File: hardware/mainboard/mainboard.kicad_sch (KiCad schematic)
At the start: 124 parts, among them J1 USB 2.0, J10 EXP1, J11 EXP2, J23 JST XH, J24 JST XH, J25 JST XH, J26 JST XH, J27 JST XH, J3 JST XH, J4 JST XH, J5 JST XH, J6 JST XH, J9 Power In, Q1 AGM308MBP, SW13 SW_SPDT, SW14 SW_SPDT, SW2 Reset, SW9 SW_SPDT, U1 STM32F407VGTx, U11 LM5160A, U12 CD40109B, U13 CD40109B, U14 LTV-357T, U15 AMS1117-3.3, U8 LM5160A, U9 CD40109B, Y1 12 MHz

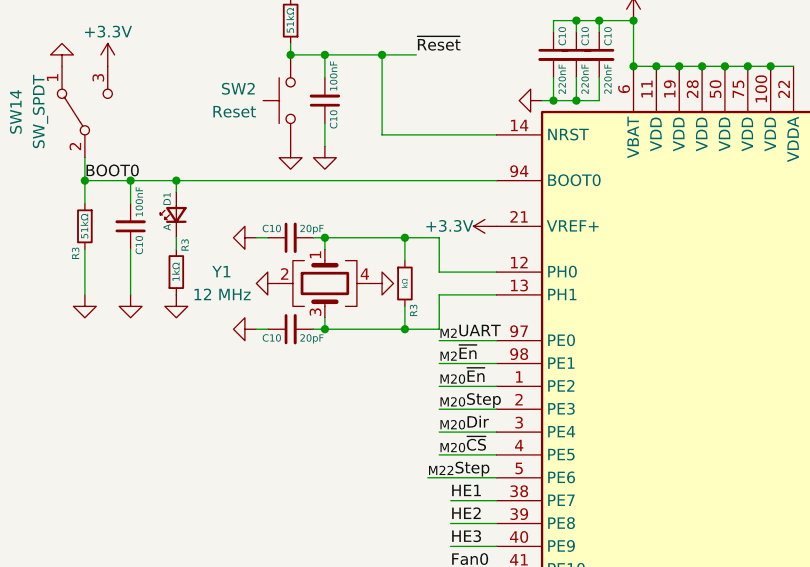
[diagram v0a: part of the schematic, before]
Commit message: test new gitignore with completed mainboard
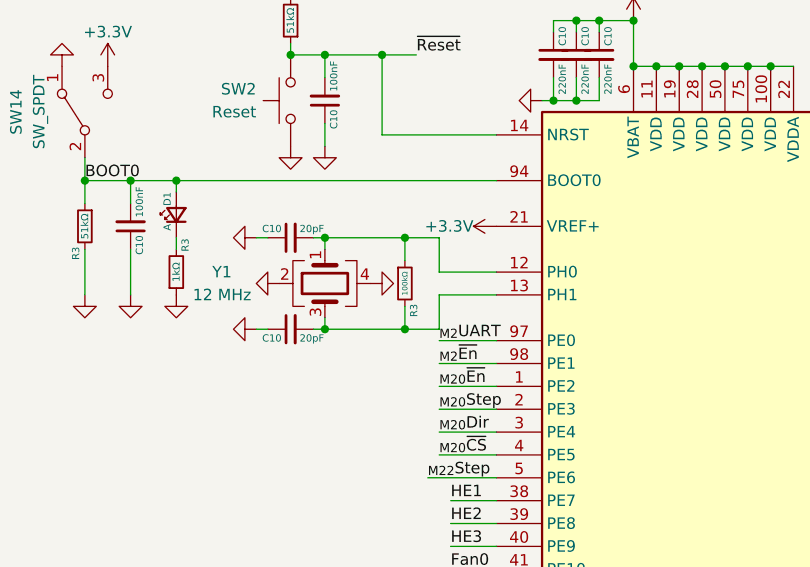
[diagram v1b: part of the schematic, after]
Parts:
- R3: value kΩ -> 100kΩ
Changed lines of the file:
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@@
       (effects (font (size 0.8 0.8)) (justify right))
     )
-    (property "Value" "kΩ" (at 153.67 73.66 90)
+    (property "Value" "100kΩ" (at 153.67 73.66 90)
       (effects (font (size 0.6 0.6)))
     )
